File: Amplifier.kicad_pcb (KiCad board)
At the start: 2 copper layers, 55.4 x 27.7 mm, 22 parts, among them Q1 BC547, Q2 2N3904

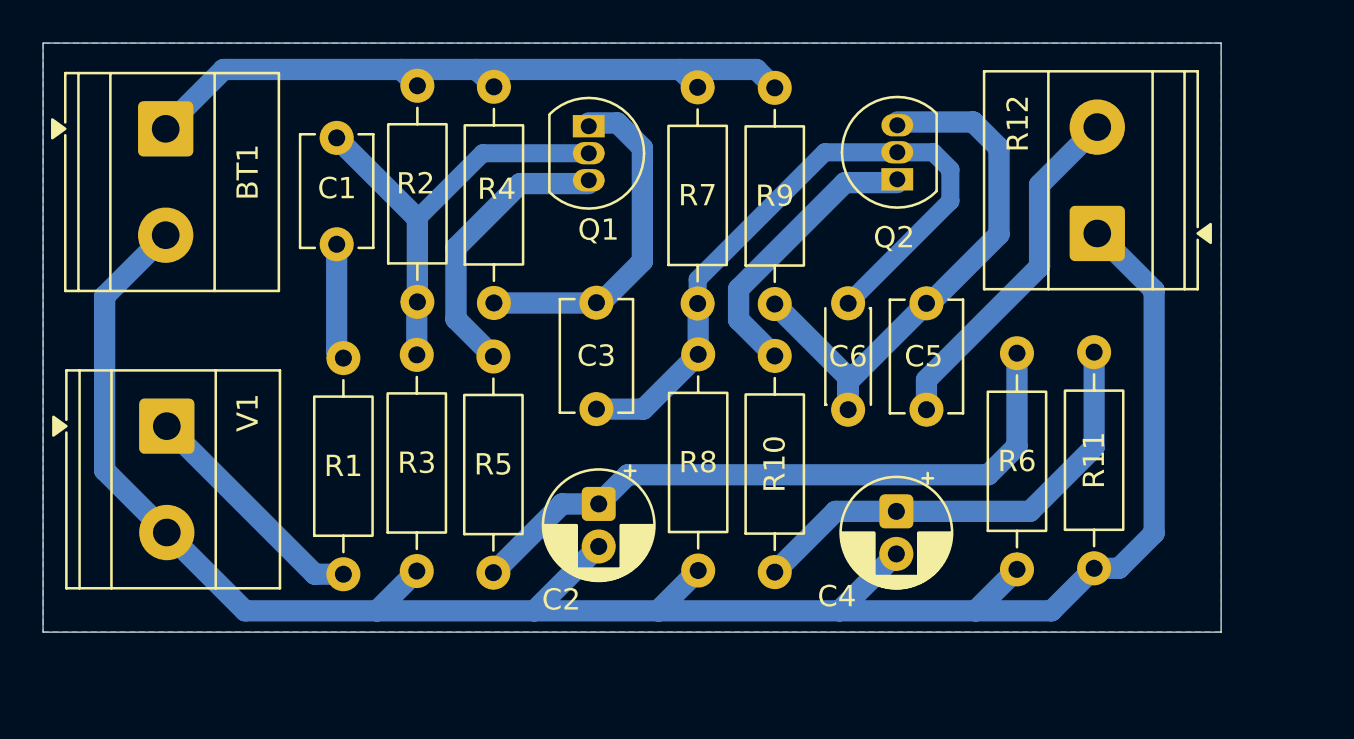
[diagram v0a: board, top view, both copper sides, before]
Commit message: v2.0 3.24.2026
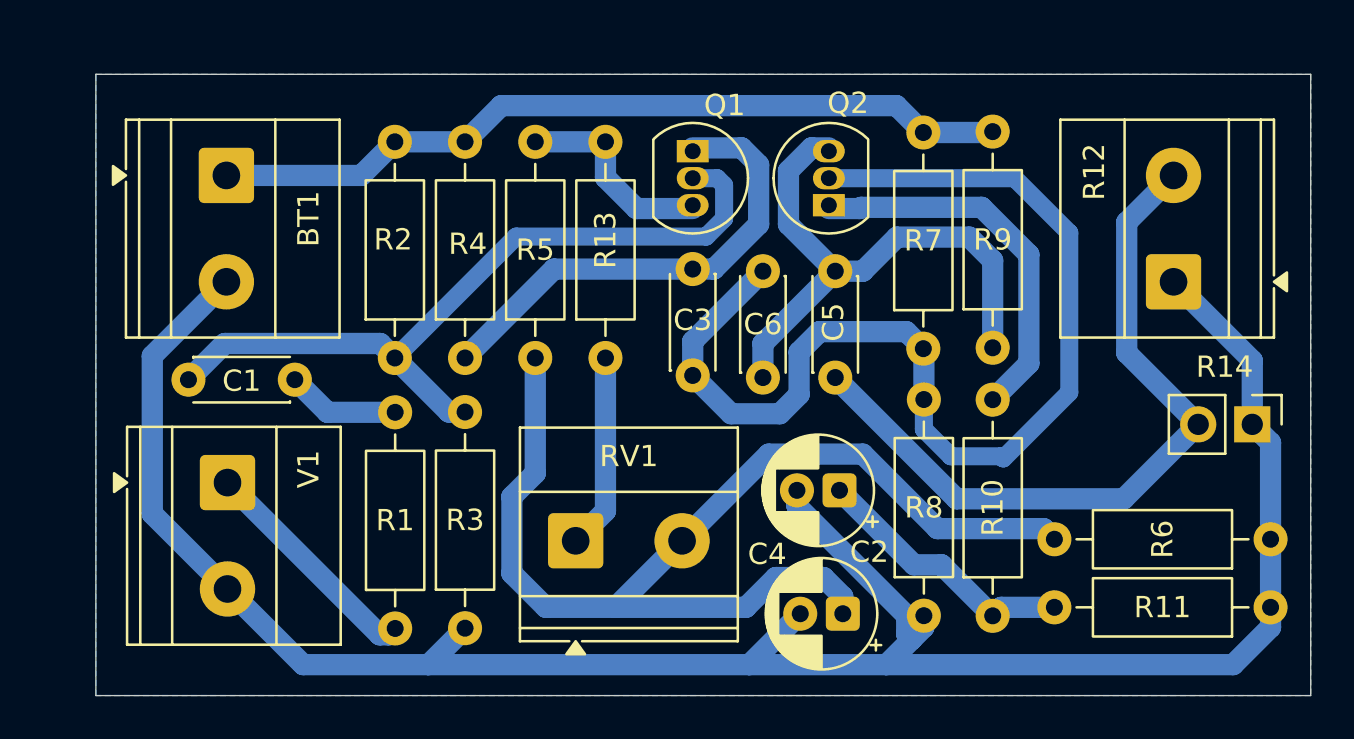
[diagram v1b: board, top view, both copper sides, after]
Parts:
- added R13: 220R, Resistor_THT:R_Axial_DIN0207_L6.3mm_D2.5mm_P10.16mm_Horizontal, F.Cu at (97.5, 64.2)
- added R14: 4K7_Pinhead, Connector_PinHeader_2.54mm:PinHeader_1x02_P2.54mm_Vertical, F.Cu at (127.9, 67.4)
- added RV1: R_Potentiometer, TerminalBlock_Phoenix:TerminalBlock_Phoenix_MKDS-1,5-2_1x02_P5.00mm_Horizontal, F.Cu at (96.1, 72.8)
- C1, C3, C5: footprint Capacitor_THT:C_Disc_D5.1mm_W3.2mm_P5.00mm -> Capacitor_THT:C_Disc_D4.3mm_W1.9mm_P5.00mm
- C2, C4: value 30 uF -> 33 uF
- C6: value 180 uF -> 150 pF
- R1: value 50R -> 51R
- R11: value 2K85 -> 2K7
- R12: value 4K7 -> 4K7_TerminalBlock
- R2: value 25K -> 24K
- R3: value 4K5 -> 4K7
- R6: value 350R -> 330R
- R8: value 55K -> 56K
- R9: value 6K -> 6K2
- moved C2 12.6 mm to (108.6, 76.3), turned to 180 degrees
- moved R6 12.0 mm to (128.7, 72.8), turned to 180 degrees
- moved R7 10.8 mm to (112.4, 63.8)
- moved R8 10.8 mm to (112.4, 76.3)
- moved R10 10.4 mm to (115.7, 76.4)
- moved R9 10.4 mm to (115.7, 63.8)
- moved R5 10.3 mm to (94.2, 64.2)
- moved R11 8.49 mm to (128.7, 76.0), turned to 180 degrees
- moved C1 6.66 mm to (82.9, 65.3), turned to 180 degrees
- moved Q1 5.02 mm to (101.6, 54.5)
- moved C3 4.79 mm to (101.6, 60.1)
- moved C5 4.55 mm to (108.3, 65.2)
- moved C6 4.28 mm to (104.9, 65.2)
- moved R12 4.24 mm to (124.2, 60.7)
- moved V1 3.90 mm to (79.7, 70.1)
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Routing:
- net Net-(C2-Pad1): track 31.4 -> 53.8 mm
- net Net-(Q2-B): track 32.4 -> 53.3 mm
- net Net-(C5-Pad1): track 16.6 -> 34.9 mm
- net Net-(Q1-B): track 21.1 -> 36.4 mm
- net Net-(C4-Pad1): track 21.9 -> 12.7 mm
- net Net-(R13-Pad1): track 0.00 -> 9.17 mm
- net GND: track 97.1 -> 105.6 mm
- net Net-(Q1-C): track 16.1 -> 22.6 mm
- net Net-(Q2-E): track 13.4 -> 17.9 mm
- net Net-(BT1-+): track 33.6 -> 37.9 mm
- net Net-(Q1-E): track 13.3 -> 9.68 mm
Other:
- board size 55.4 x 27.7 mm -> 57.1 x 29.2 mm
